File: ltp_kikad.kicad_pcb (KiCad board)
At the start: 2 copper layers, 65 x 56.5 mm, 22 parts, among them IC1 SamacSys_Parts_HT16K33-28SOP, IC2 SamacSys_Parts_HT16K33-28SOP, J2 RPi_GPIO

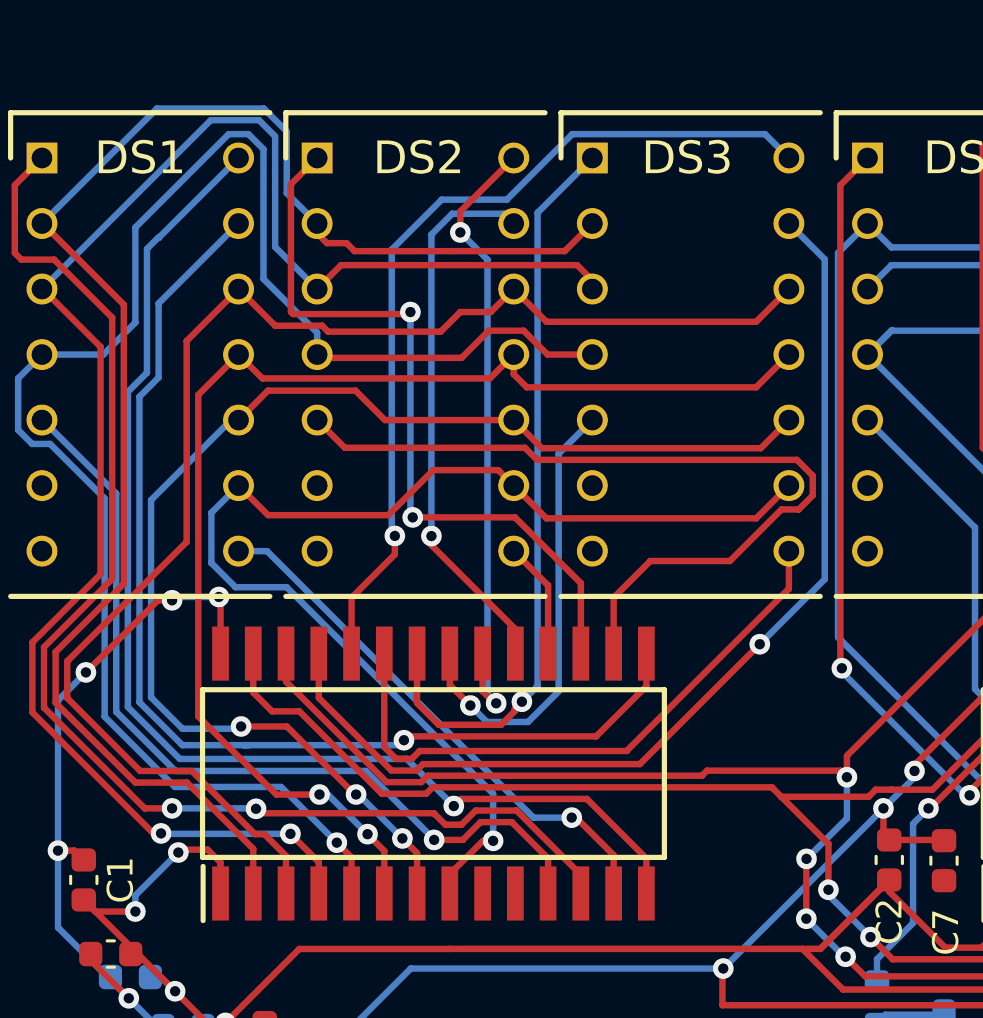
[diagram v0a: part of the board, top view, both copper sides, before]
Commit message: Minor improvements
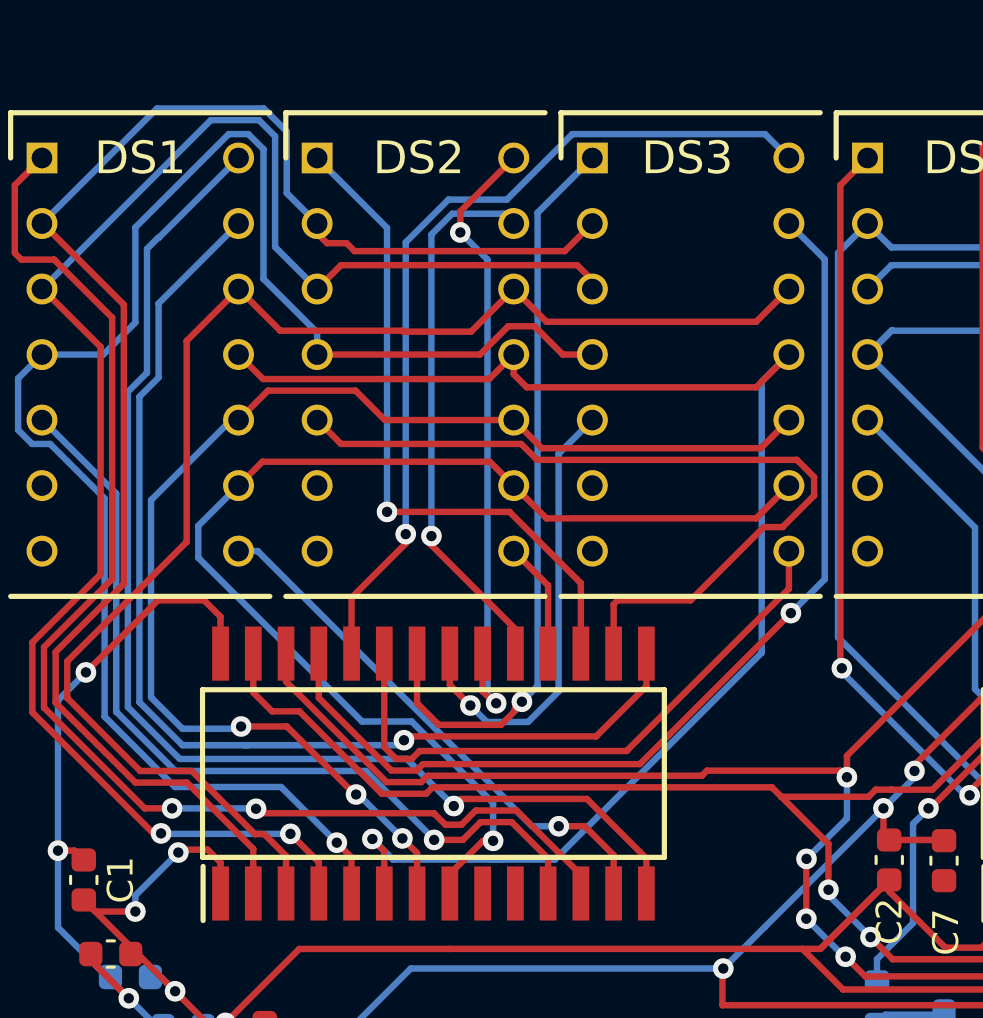
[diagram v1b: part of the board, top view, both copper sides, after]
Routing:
- net ca4: track 49.3 -> 57.2 mm, vias 2 -> 1
- net an8: track 29.4 -> 26.2 mm, vias 2 -> 1
- net +5V: track 110.4 -> 109.8 mm, vias 9 -> 7
